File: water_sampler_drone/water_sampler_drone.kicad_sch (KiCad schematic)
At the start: 6 parts, among them M1 Stepper_Motor_bipolar, M2 Motor_DC, U1 Ultrasonic Sensor, U2 Step Motor Driver, U3 H Bridge

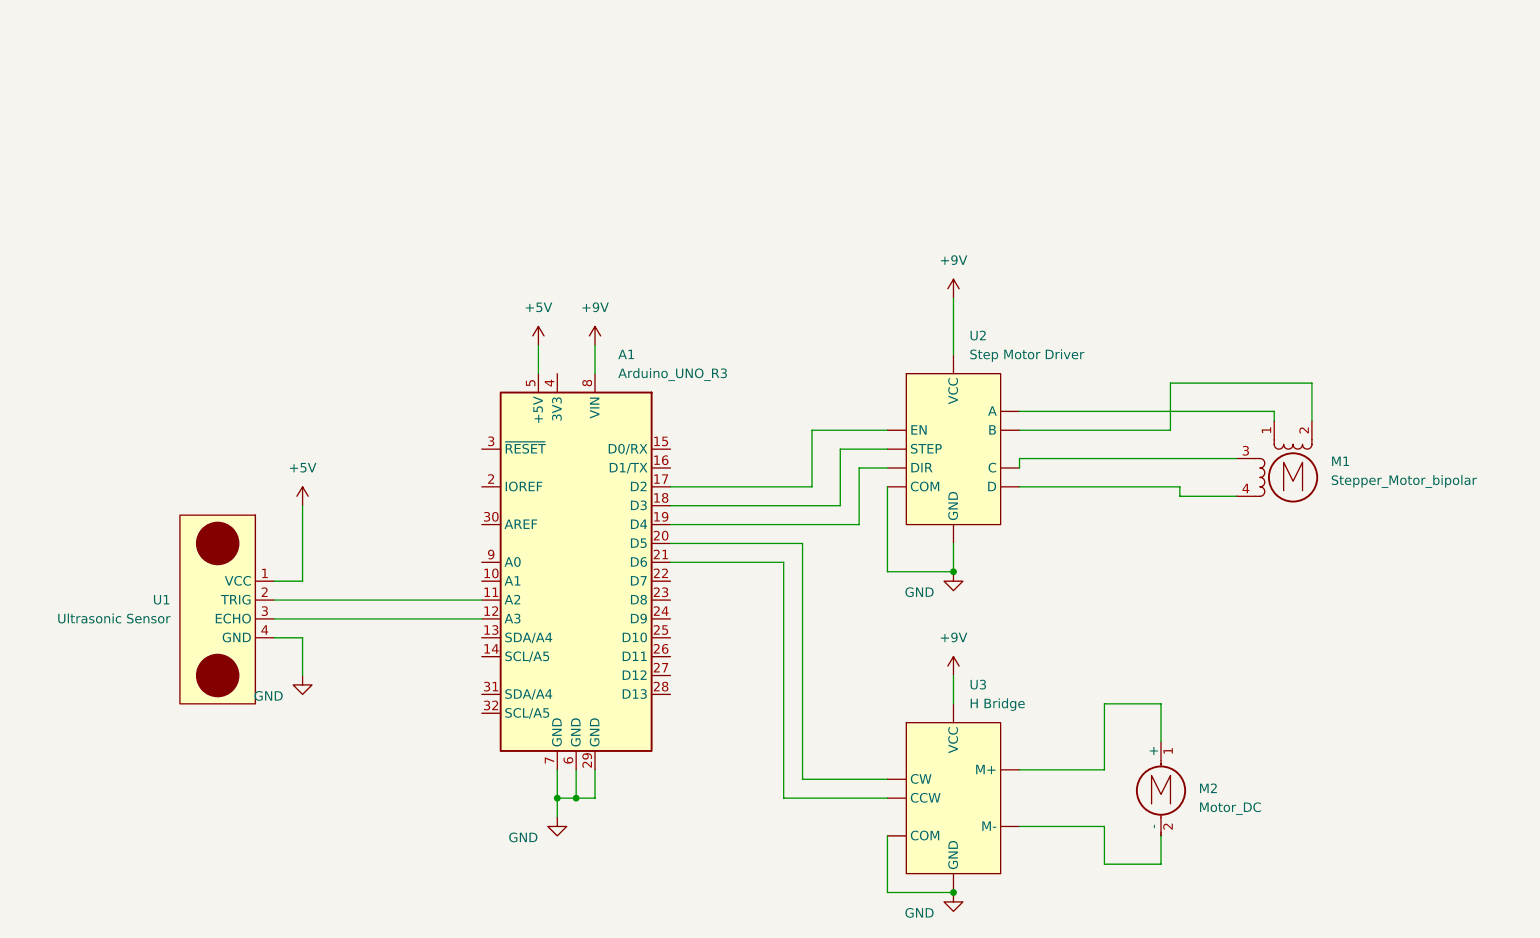
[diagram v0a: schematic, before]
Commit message: update water sampler
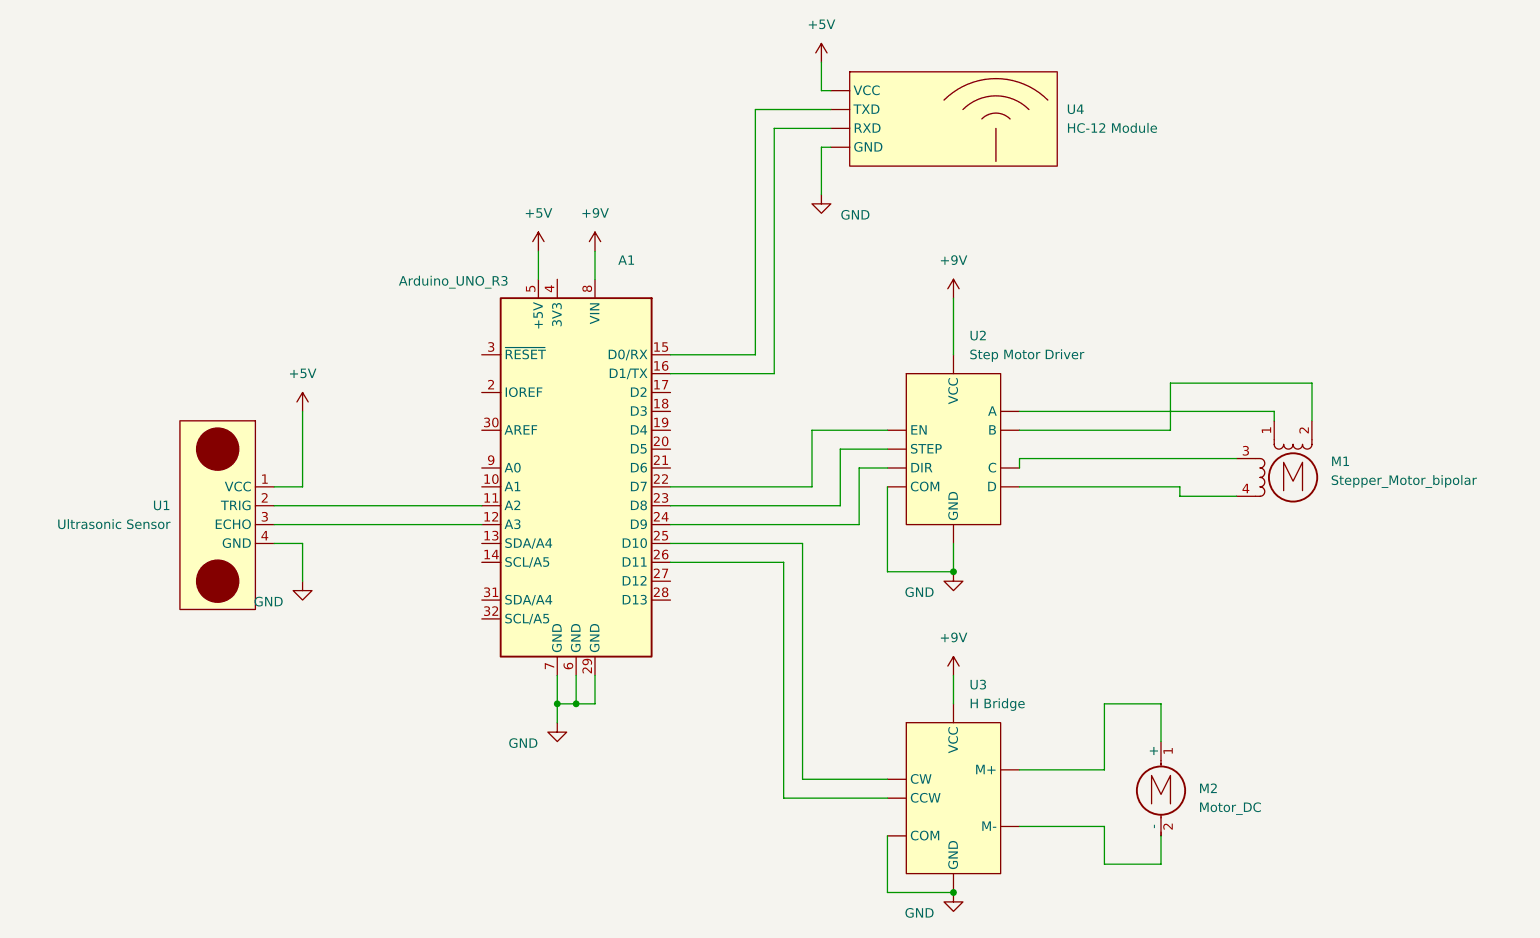
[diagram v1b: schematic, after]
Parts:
- added U4: HC-12 Module, symbol AA_parts:HC-12_Mod
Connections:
- net +5V: now also U4. (GND)
- net GND: now also U4. (GND)
- net at A1.20 (D5): no longer U3. (M-)
- net at A1.21 (D6): no longer U3. (M-)
- net at A1.15 (D0/RX): now also U4. (GND)
- net at A1.16 (D1/TX): now also U4. (GND)
- net at A1.17 (D2): no longer U2. (D)
- net at A1.18 (D3): no longer U2. (D)
- net at A1.19 (D4): no longer U2. (D)
- net at A1.22 (D7): now also U2. (D)
- net at A1.23 (D8): now also U2. (D)
- net at A1.24 (D9): now also U2. (D)
- net at A1.25 (D10): now also U3. (M-)
- net at A1.26 (D11): now also U3. (M-)
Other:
- moved on the sheet: A1, U1
